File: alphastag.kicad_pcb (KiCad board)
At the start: 2 copper layers, 221.5 x 102.4 mm, 89 parts, among them SW1 SW_Push, U1 SRV05-4, U2 ATmega32U4-A, Y1 16MHz

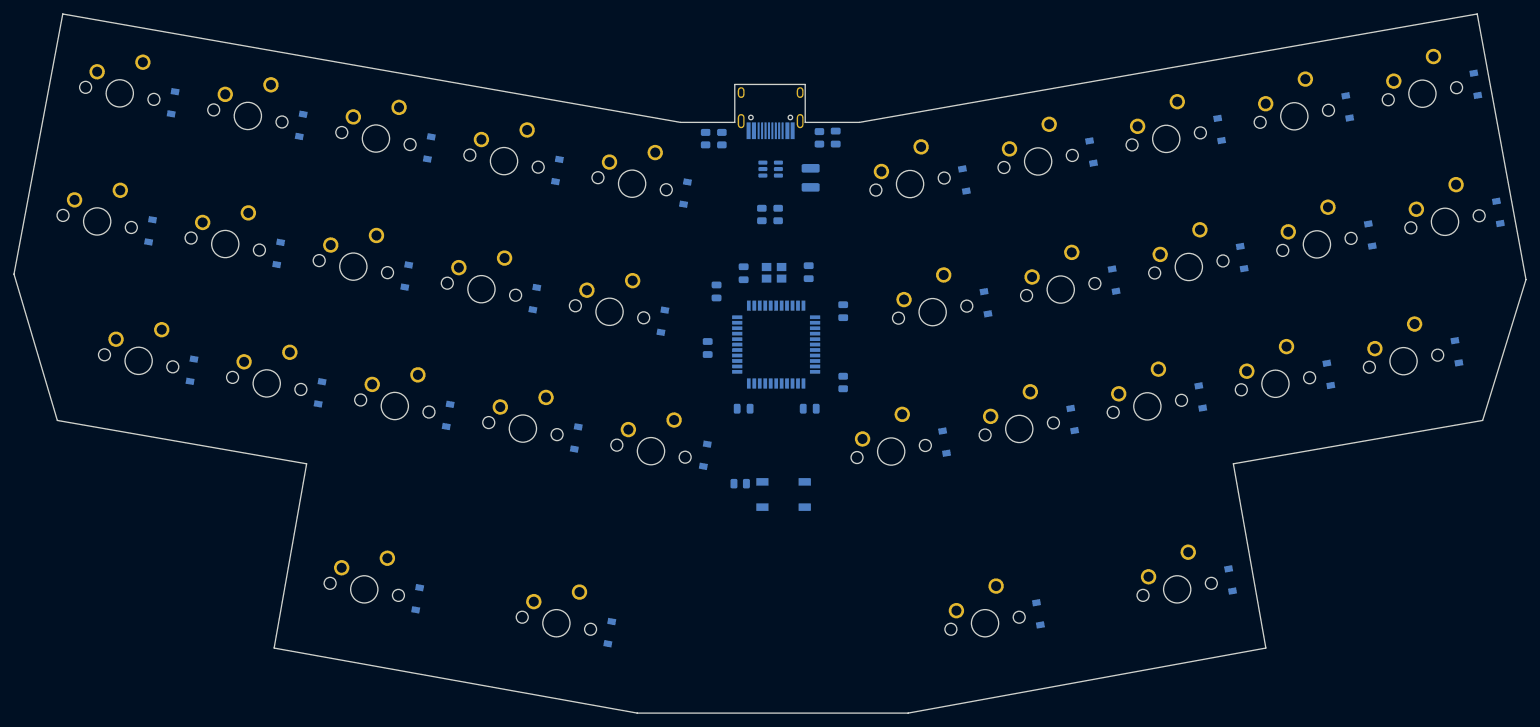
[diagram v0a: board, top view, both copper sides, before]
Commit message: routing
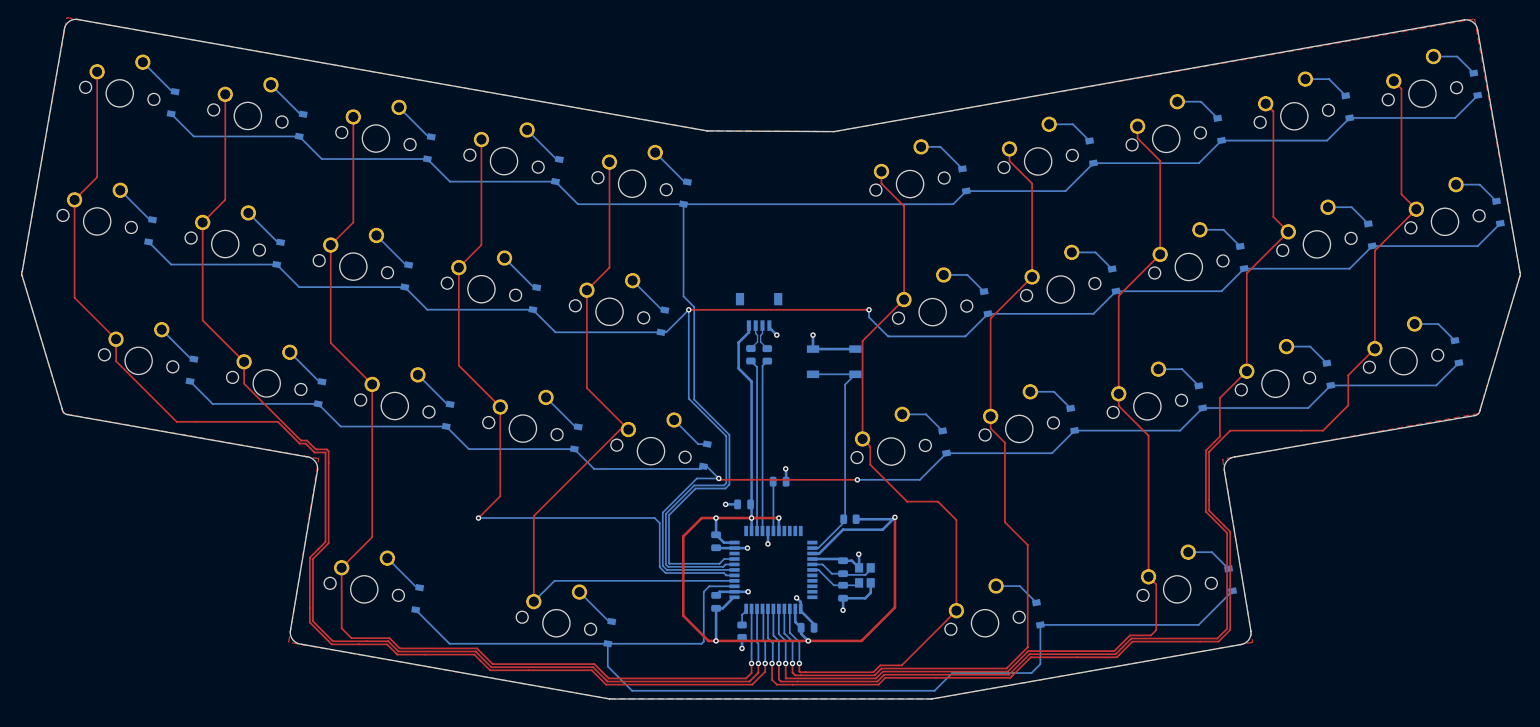
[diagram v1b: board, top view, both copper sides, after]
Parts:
- removed C3: 4.7uF, Capacitor_SMD:C_0805_2012Metric
- removed F1: Polyfuse_Small, Fuse:Fuse_1210_3225Metric
- removed U1: SRV05-4, Package_TO_SOT_SMD:SOT-23-6
- removed UR1: 1M, Resistor_SMD:R_0805_2012Metric
- removed UR2, UR3: 5.1k, Resistor_SMD:R_0805_2012Metric
- removed USB1: HRO-TYPE-C-31-M-12, Type-C:HRO-TYPE-C-31-M-12-HandSoldering
- added J1: Conn_01x04_Female, random-keyboard-parts:JST-SR-4, B.Cu at (125.8, 56.7)
- moved C1 47.1 mm to (138.1, 100.5), turned to 90 degrees
- moved C6 46.7 mm to (132.9, 105.8), turned to 0 degrees
- moved Y1 46.3 mm to (141.3, 98.1), turned to 90 degrees
- moved C2 45.5 mm to (138.1, 96.9), turned to -90 degrees
- moved R4 39.3 mm to (123.3, 106.3)
- moved C5 36.6 mm to (119.5, 93.1), turned to -90 degrees
- moved U2 33.0 mm to (127.9, 97.3), turned to -90 degrees
- moved C7 31.4 mm to (119.5, 102.0), turned to 90 degrees
- moved C4 22.2 mm to (128.8, 84.4), turned to 0 degrees
- moved SW1 20.8 mm to (136.8, 66.8), turned to 180 degrees
- moved R2 20.6 mm to (127.0, 65.8)
- moved R3 20.6 mm to (124.6, 65.8)
- moved R1 16.9 mm to (139.1, 89.9), turned to 0 degrees
- moved C8 14.0 mm to (123.6, 87.7), turned to 180 degrees
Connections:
- D31 pad 1: unconnected-(D31-Pad1) -> /ROW3
- R2 pad 1: D+ -> /D+
- R3 pad 1: D- -> /D-
- U2 pad 10: /ROW1 -> unconnected-(U2-Pad10)
- U2 pad 11: /ROW0 -> unconnected-(U2-Pad11)
- U2 pad 25: unconnected-(U2-Pad25) -> /COL5
- U2 pad 26: unconnected-(U2-Pad26) -> /COL6
- U2 pad 27: unconnected-(U2-Pad27) -> /COL7
- U2 pad 28: unconnected-(U2-Pad28) -> /COL8
- U2 pad 29: unconnected-(U2-Pad29) -> /COL9
- U2 pad 30: unconnected-(U2-Pad30) -> /COL0
- U2 pad 31: unconnected-(U2-Pad31) -> /COL1
- U2 pad 32: unconnected-(U2-Pad32) -> /COL2
- U2 pad 36: unconnected-(U2-Pad36) -> /ROW3
- U2 pad 37: unconnected-(U2-Pad37) -> /COL4
- U2 pad 38: unconnected-(U2-Pad38) -> /COL3
- U2 pad 39: unconnected-(U2-Pad39) -> /ROW2
- U2 pad 40: unconnected-(U2-Pad40) -> /ROW1
- U2 pad 41: unconnected-(U2-Pad41) -> /ROW0
- U2 pad 8: /ROW3 -> unconnected-(U2-Pad8)
- U2 pad 9: /ROW2 -> unconnected-(U2-Pad9)
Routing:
- net /ROW0: track 0.00 -> 274.9 mm
- net /ROW1: track 0.00 -> 270.1 mm, vias 0 -> 2
- net /ROW2: track 0.00 -> 228.0 mm, vias 0 -> 2
- net /COL0: track 0.00 -> 189.0 mm, vias 0 -> 1
- net /COL9: track 0.00 -> 185.0 mm, vias 0 -> 1
- net /COL1: track 0.00 -> 167.5 mm, vias 0 -> 1
- net /COL8: track 0.00 -> 164.2 mm, vias 0 -> 1
- net /ROW3: track 0.00 -> 162.2 mm
- net /COL2: track 0.00 -> 153.4 mm, vias 0 -> 1
- net /COL7: track 0.00 -> 147.8 mm, vias 0 -> 1
- net +5V: track 0.00 -> 147.3 mm, vias 0 -> 6
- net /COL6: track 0.00 -> 125.3 mm, vias 0 -> 1
- net /COL5: track 0.00 -> 113.1 mm, vias 0 -> 1
- net /COL3: track 0.00 -> 105.4 mm, vias 0 -> 1
- net /COL4: track 0.00 -> 105.3 mm
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- added copper zone on F.Cu, net GND
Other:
- board size 221.5 x 102.4 mm -> 219.5 x 99.5 mm
